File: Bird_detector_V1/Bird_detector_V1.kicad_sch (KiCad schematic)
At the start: 0 parts

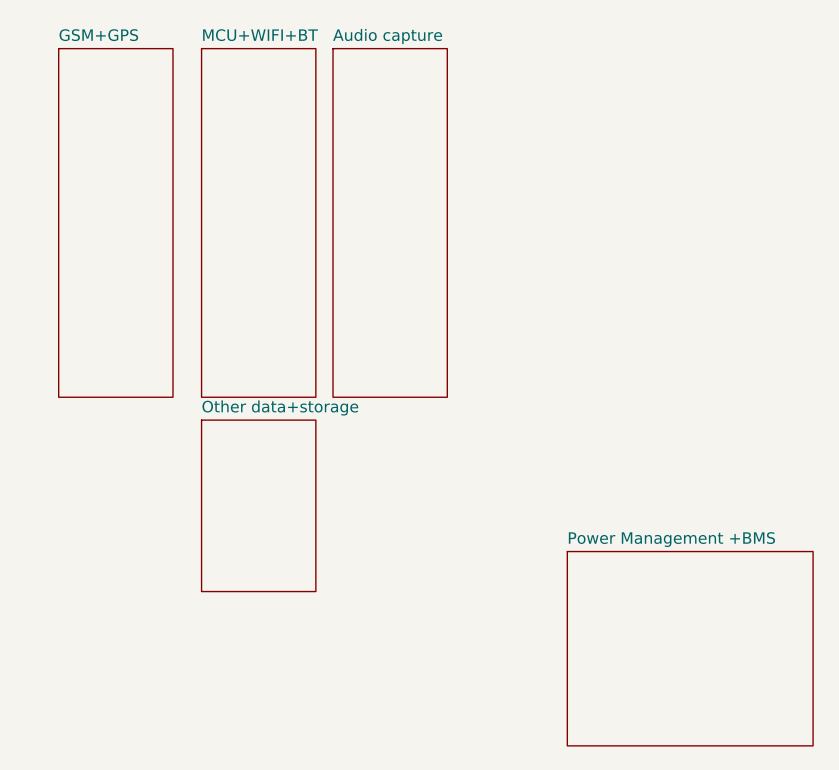
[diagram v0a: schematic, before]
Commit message: r
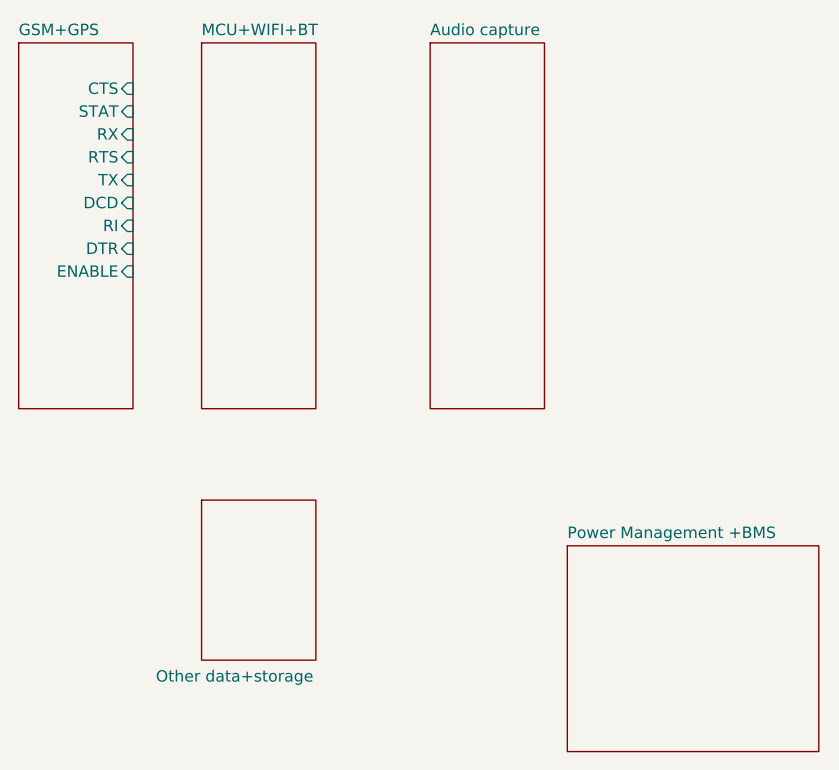
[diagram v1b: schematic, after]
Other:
- sheet GSM+GPS ports: added CTS, DCD, DTR, ENABLE, RI, RTS, RX, STAT, TX; removed none
